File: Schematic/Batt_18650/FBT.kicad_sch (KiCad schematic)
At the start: 17 parts, among them J1 TRRS Connector 3.5, J2 Conn_01x04, SW1 SW_SPDT

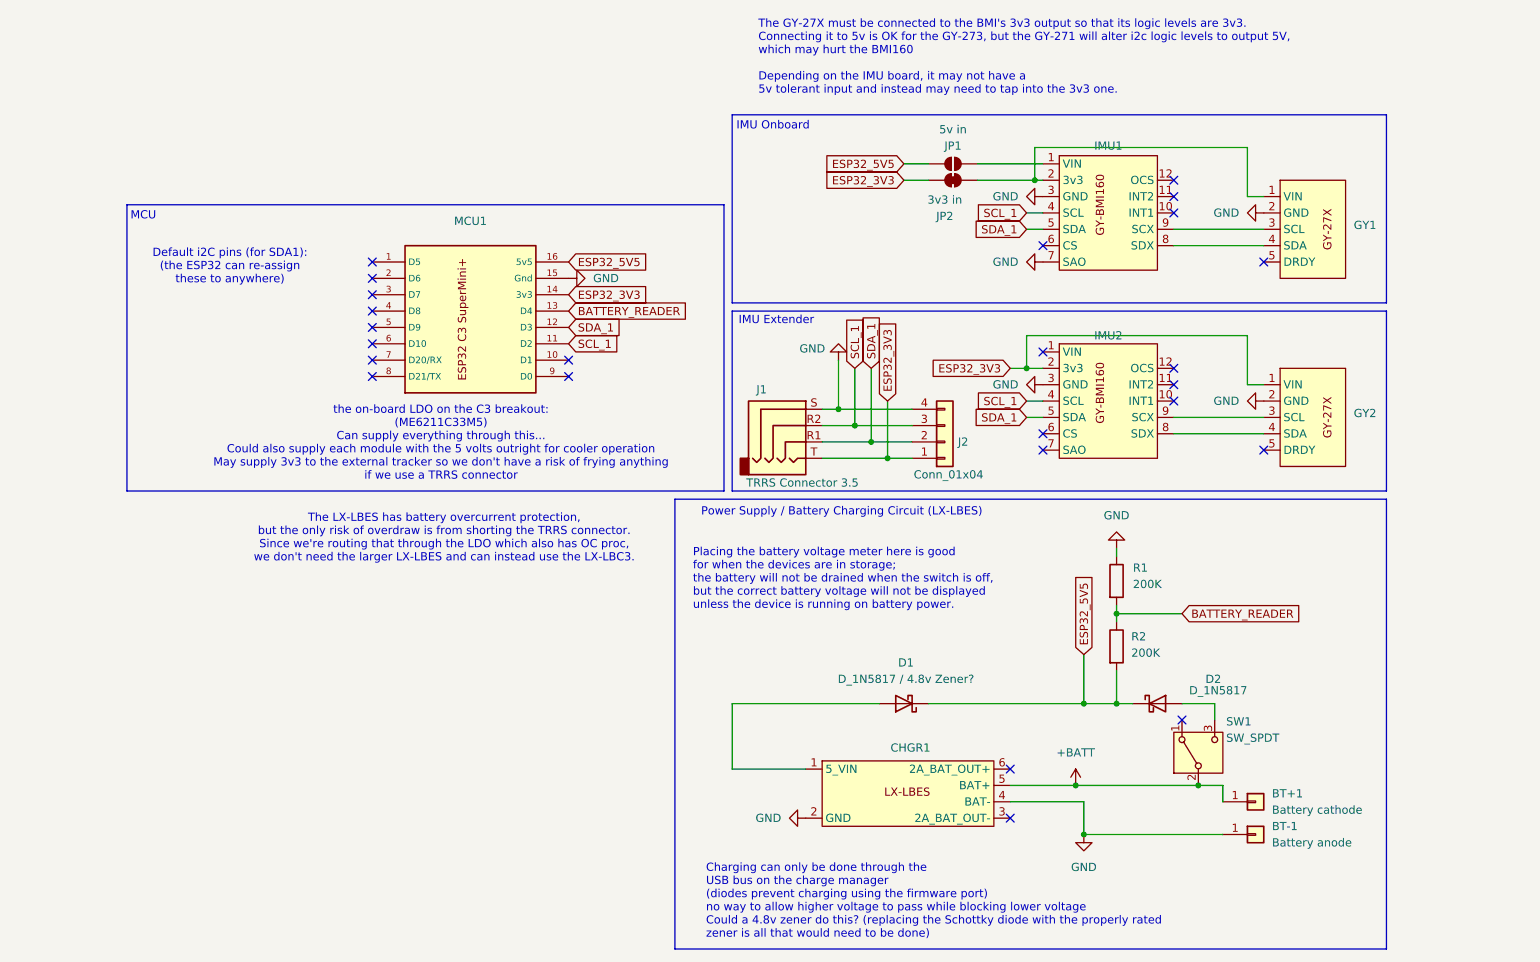
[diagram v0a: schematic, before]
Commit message: work on PCBs, logos, and case
did more work on 18650 battery model
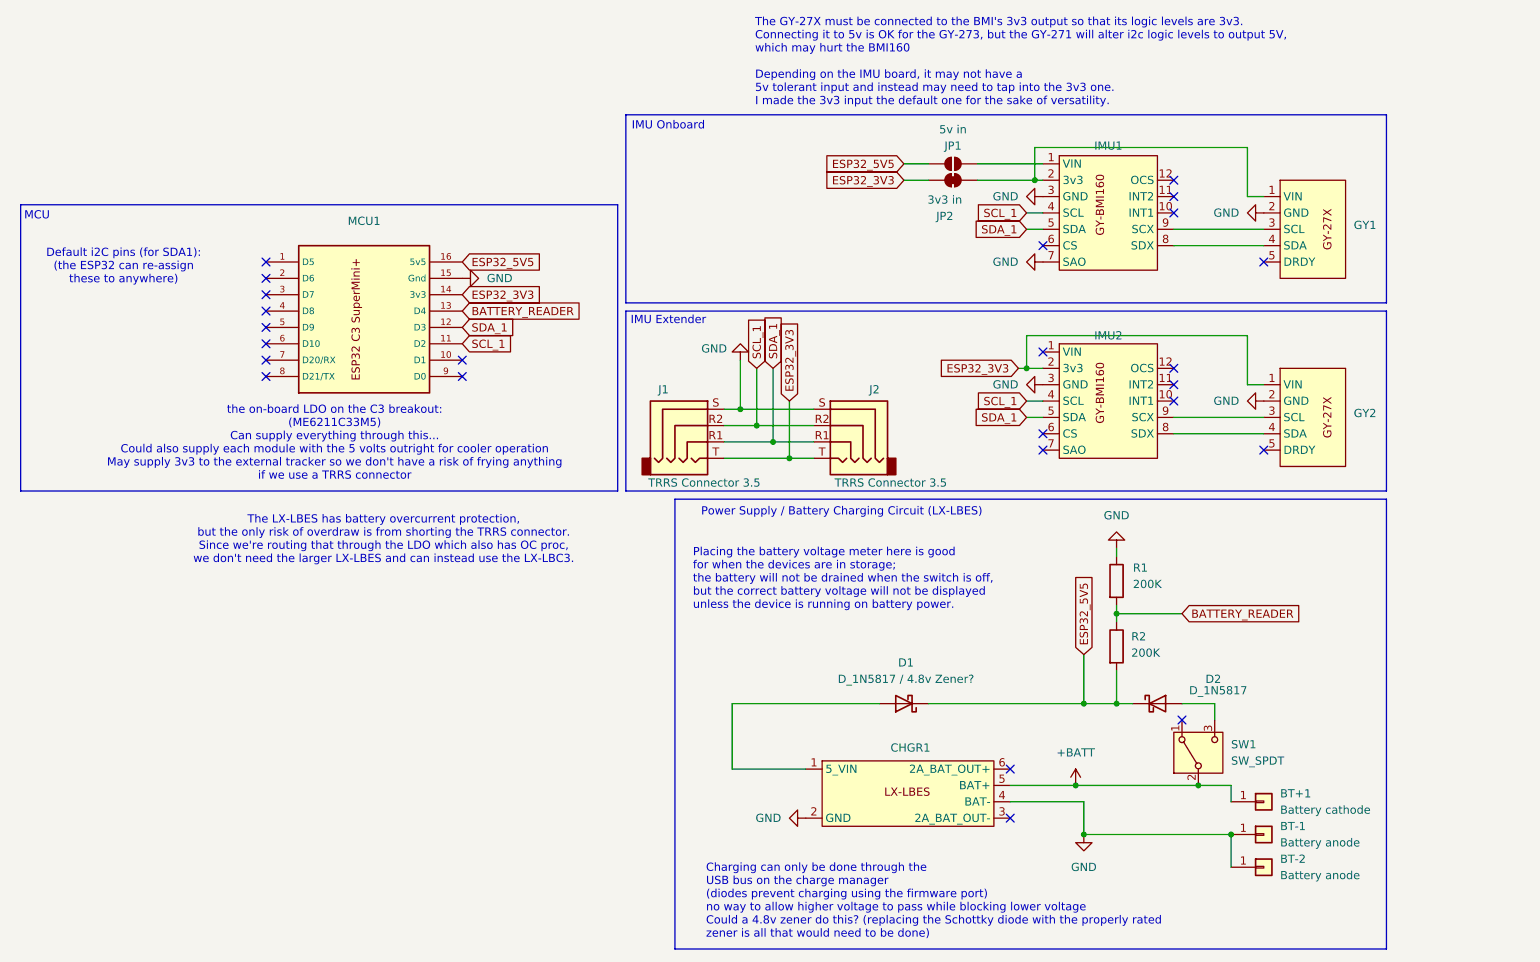
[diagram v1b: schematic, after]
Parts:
- removed J2: Conn_01x04, Connector_JST:JST_PH_S4B-PH-K_1x04_P2.00mm_Horizontal, symbol Connector_Generic:Conn_01x04
- added BT-2: Battery anode, Connector_PinHeader_2.54mm:PinHeader_1x01_P2.54mm_Vertical, symbol Connector_Generic:Conn_01x01
- added J2: TRRS Connector 3.5, My_Library:PJ-320A, symbol Connector_Audio:AudioJack4
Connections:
- net ESP32_3V3: now also J2.T
- net GND: now also BT-2.1 (Pin_1), J2.S
- net SCL_1: now also J2.R2
- net SDA_1: now also J2.R1
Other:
- note added: "The GY-27X must be connected to the BMI's 3v3 output so that its logic levels are 3v3. Connecting it to 5v is OK for the GY-273, but the GY-271 will alter i2c logic levels to output 5V, which may hurt the BMI160 Depending on the IMU board, it may not have a 5v tolerant input and instead may need to tap into the 3v3 one. I made the 3v3 input the default one for the sake of versatility."
- note removed: "The GY-27X must be connected to the BMI's 3v3 output so that its logic levels are 3v3. Connecting it to 5v is OK for the GY-273, but the GY-271 will alter i2c logic levels to output 5V, which may hurt the BMI160 Depending on the IMU board, it may not have a 5v tolerant input and instead may need to tap into the 3v3 one."
- moved on the sheet: J1, MCU1
